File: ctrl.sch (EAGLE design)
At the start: 47 parts, among them U1 TPS92513, U2 TPS92513

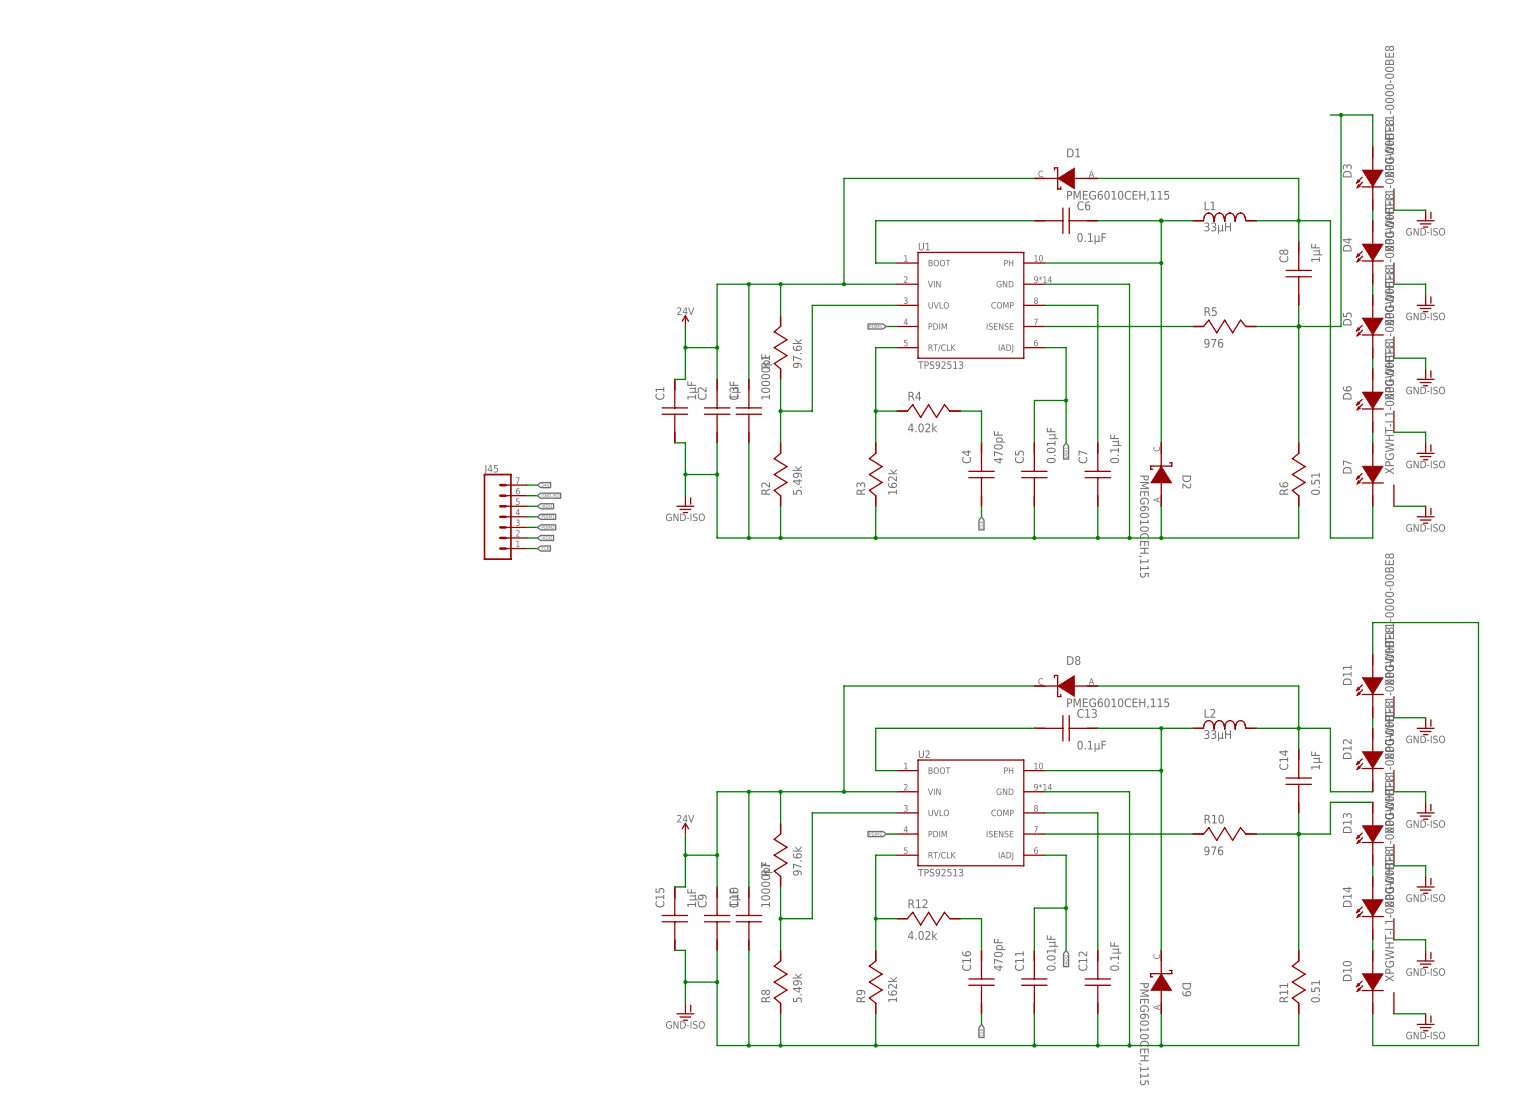
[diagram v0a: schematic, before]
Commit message: save
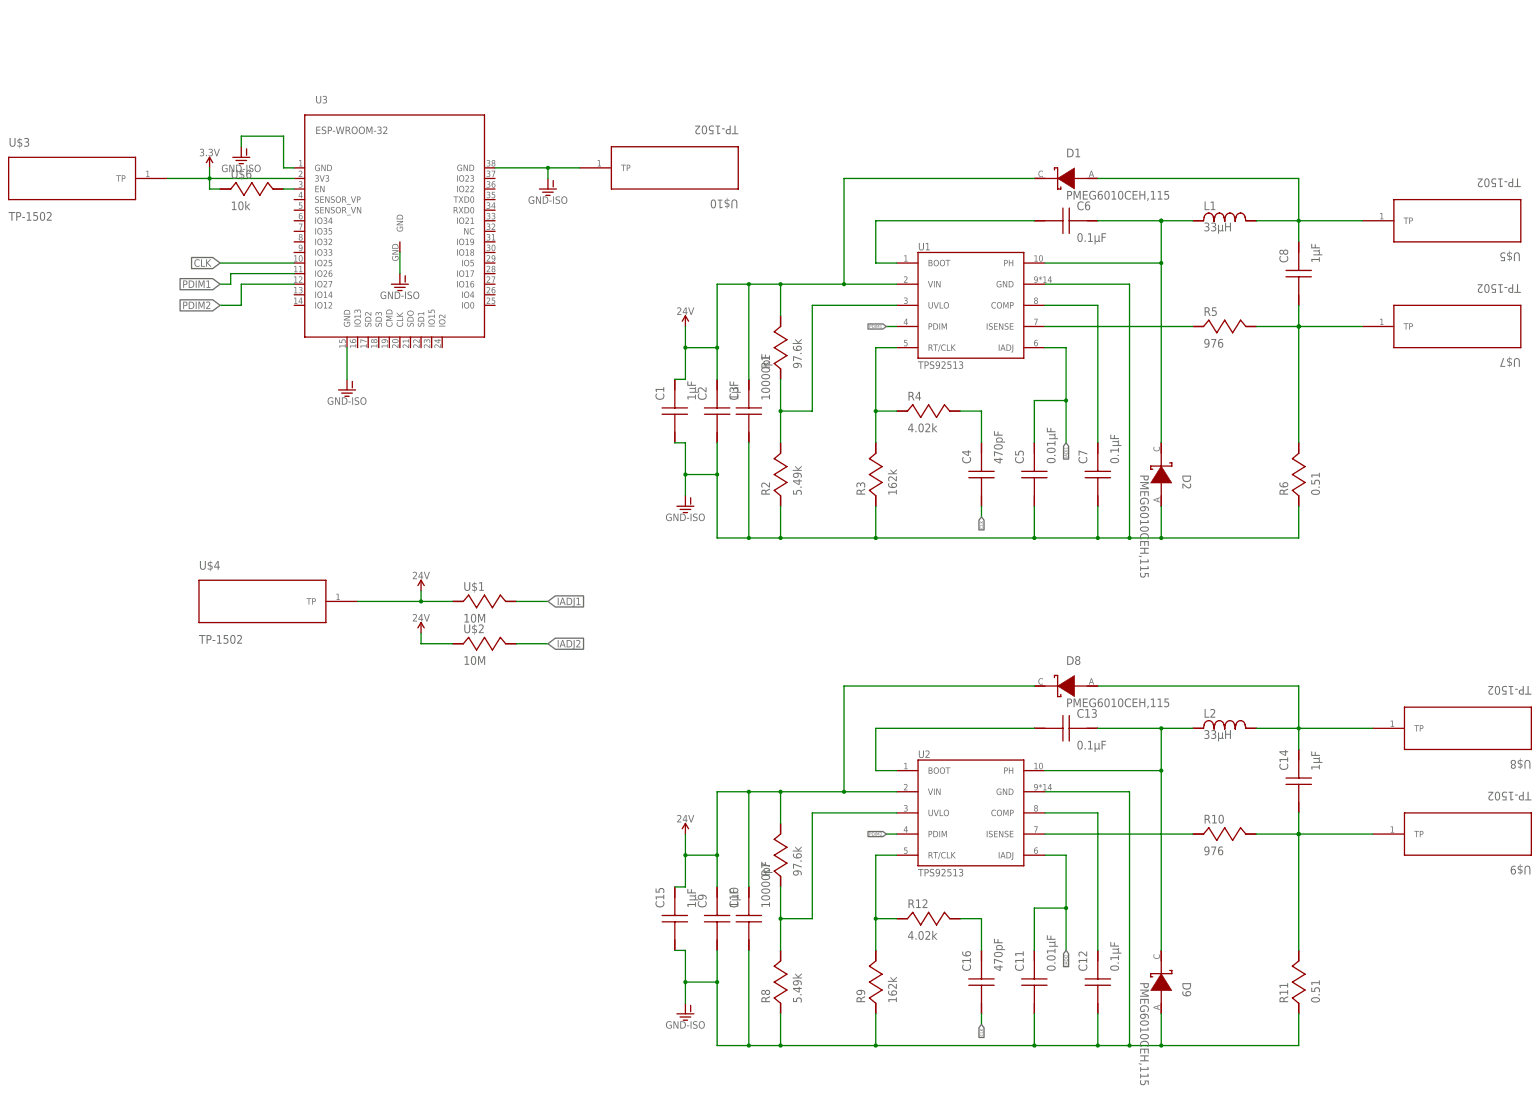
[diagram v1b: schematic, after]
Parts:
- removed D10, D11, D12, D13, D14, D3, D4, D5, D6, D7: XPGWHT-L1-0000-00BE8, derek:XPGWHT-L1-0000-00BE8
- removed J45: (no value), derek:CONN_07NO_SILK
- added U$1, U$2: 10M, derek:CRCW040210M0JNED
- added U$10, U$3, U$4, U$5, U$7, U$8, U$9: TP-1502, derek:TP-1502
- added U$6: 10k, derek:CRCW060310K0FKEA
- added U3: ESP-WROOM-32, derek:ESP-WROOM-32
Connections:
- removed net N$12: D6.C, D7.A
- removed net N$13: D3.C, D4.A
- removed net N$14: D4.C, D5.A
- removed net N$15: D5.C, D6.A
- removed net N$2: D11.C, D12.A
- removed net N$22: D13.C, D14.A
- removed net N$24: D10.A, D14.C
- removed net N$27: D10.C, D11.A
- new net 3.3V: U$3.TP, U$6.2, U3.3V3
- new net N$29: U$6.1, U3.EN
- net 24V: now also U$1.2, U$2.2, U$4.TP; no longer J45.7
- net CLK: now also U3.IO25; no longer J45.1
- net GND-ISO: now also U$10.TP, U3.GND, U3.GND@1, U3.GND@15, U3.GND@38; no longer D10.GND, D11.GND, D12.GND, D13.GND, D14.GND, D3.GND, D4.GND, D5.GND, D6.GND, D7.GND, J45.6
- net IADJ1: now also U$1.1; no longer J45.5
- net IADJ2: now also U$2.1; no longer J45.2
- net N$23: now also U$8.TP; no longer D12.C
- net N$26: now also U$9.TP; no longer D13.A
- net N$6: now also U$7.TP; no longer D3.A
- net N$7: now also U$5.TP; no longer D7.C
- net PDIM1: now also U3.IO26; no longer J45.4
- net PDIM2: now also U3.IO27; no longer J45.3
